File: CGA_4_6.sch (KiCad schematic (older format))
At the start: 3 parts, among them U1 74S112, U26 74S04, U47 74LS51

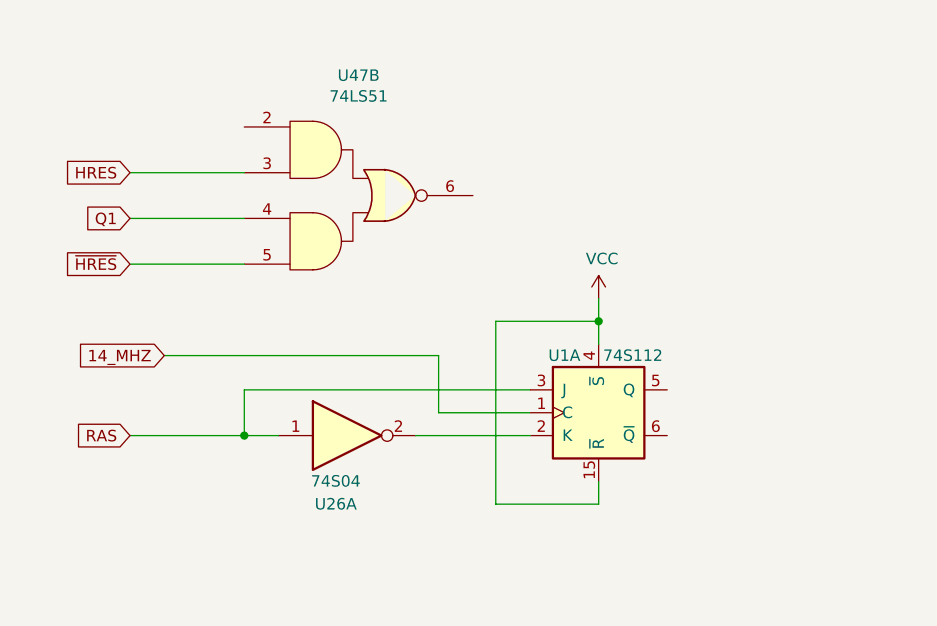
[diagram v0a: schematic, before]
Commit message: More CGA sheet 4
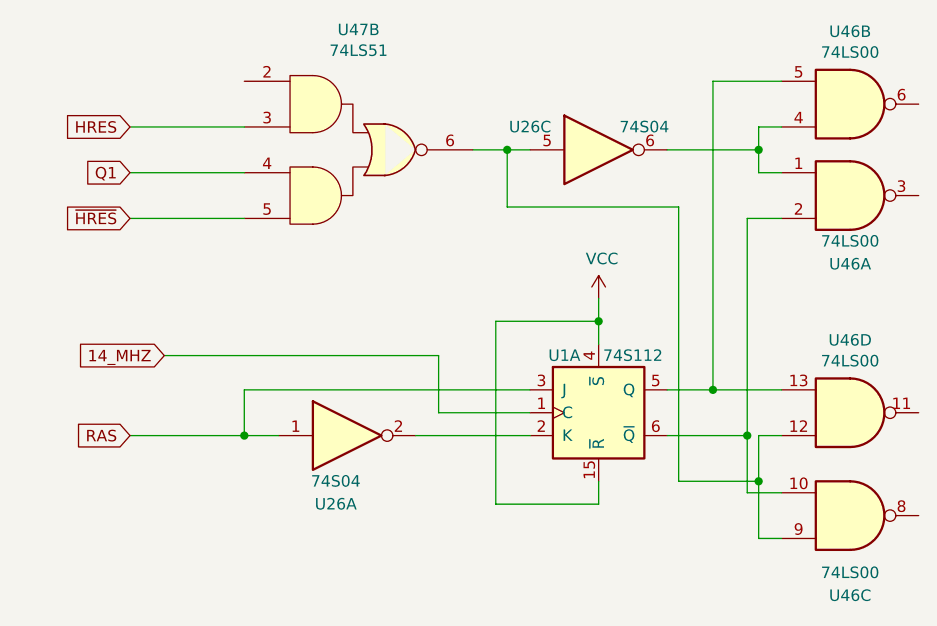
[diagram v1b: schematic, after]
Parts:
- added unit 3 of U26
- added U46: 74LS00, Package_DIP:DIP-14_W7.62mm_LongPads, symbol 74xx:74LS00
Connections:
- net at U47.6: now also U26.5, U46.12, U46.9
- net at U1.5 (Q): now also U46.13, U46.5
- net at U1.6 (~Q): now also U46.10, U46.2
- new net: U26.6, U46.1, U46.4
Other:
- moved on the sheet: U47B
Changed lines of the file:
@@
 L 74xx:74LS51 U47
 U 2 1 62D15655
-P 1850 1400
-F 0 "U47" H 1850 1925 50  0000 C CNN
-F 1 "74LS51" H 1850 1834 50  0000 C CNN
-F 2 "Package_DIP:DIP-14_W7.62mm_LongPads" H 1850 1400 50  0001 C CNN
-F 3 "http://www.ti.com/lit/ds/symlink/sn74ls51.pdf" H 1850 1400 50  0001 C CNN
-	2    1850 1400
-	1    0    0    -1
-$EndComp
+P 1850 1200
+F 0 "U47" H 1850 1725 50  0000 C CNN
+F 1 "74LS51" H 1850 1634 50  0000 C CNN
+F 2 "Package_DIP:DIP-14_W7.62mm_LongPads" H 1850 1200 50  0001 C CNN
+F 3 "http://www.ti.com/lit/ds/symlink/sn74ls51.pdf" H 1850 1200 50  0001 C CNN
+	2    1850 1200
+	1    0    0    -1
+$EndComp
+Wire Wire Line
+	1350 1100 850  1100
+Text GLabel 850  1100 0    50   Input ~ 0
+HRES
 Wire Wire Line
 	1350 1300 850  1300
 Text GLabel 850  1300 0    50   Input ~ 0
-HRES
+Q1
 Wire Wire Line
 	1350 1500 850  1500
 Text GLabel 850  1500 0    50   Input ~ 0
-Q1
-Wire Wire Line
-	1350 1700 850  1700
-Text GLabel 850  1700 0    50   Input ~ 0
 ~HRES
 $Comp
@@
 	2900 1950 2900 1850
 Connection ~ 2900 1950
+$Comp
+L 74xx:74LS04 U?
+U 3 1 62D569A0
+P 2900 1200
+AR Path="/60463C57/62D569A0" Ref="U?"  Part="2"
+AR Path="/60463CC5/62D569A0" Ref="U26"  Part="3"
+F 0 "U26" H 2600 1300 50  0000 C CNN
+F 1 "74S04" H 3100 1300 50  0000 C CNN
+F 2 "Package_DIP:DIP-14_W7.62mm_LongPads" H 2900 1200 50  0001 C CNN
+F 3 "http://www.ti.com/lit/gpn/sn74LS04" H 2900 1200 50  0001 C CNN
+	3    2900 1200
+	1    0    0    -1
+$EndComp
+Wire Wire Line
+	2350 1200 2500 1200
+$Comp
+L 74xx:74LS00 U46
+U 1 1 62D5F730
+P 4000 1400
+F 0 "U46" H 4000 1100 50  0000 C CNN
+F 1 "74LS00" H 4000 1200 50  0000 C CNN
+F 2 "Package_DIP:DIP-14_W7.62mm_LongPads" H 4000 1400 50  0001 C CNN
+F 3 "http://www.ti.com/lit/gpn/sn74ls00" H 4000 1400 50  0001 C CNN
+	1    4000 1400
+	1    0    0    -1
+$EndComp
+$Comp
+L 74xx:74LS00 U46
+U 2 1 62D5E238
+P 4000 1000
+F 0 "U46" H 4000 683 50  0000 C CNN
+F 1 "74LS00" H 4000 774 50  0000 C CNN
+F 2 "Package_DIP:DIP-14_W7.62mm_LongPads" H 4000 1000 50  0001 C CNN
+F 3 "http://www.ti.com/lit/gpn/sn74ls00" H 4000 1000 50  0001 C CNN
+	2    4000 1000
+	1    0    0    1
+$EndComp
+Wire Wire Line
+	3700 1100 3600 1100
+Wire Wire Line
+	3600 1100 3600 1200
+Wire Wire Line
+	3600 1300 3700 1300
+Wire Wire Line
+	3600 1200 3200 1200
+Connection ~ 3600 1200
+Wire Wire Line
+	3600 1200 3600 1300
+Wire Wire Line
+	3200 2250 3400 2250
+Wire Wire Line
+	3400 2250 3400 900
+Wire Wire Line
+	3400 900  3700 900
+Wire Wire Line
+	3200 2450 3550 2450
+Wire Wire Line
+	3550 2450 3550 1500
+Wire Wire Line
+	3550 1500 3700 1500
+$Comp
+L 74xx:74LS00 U46
+U 3 1 62D70773
+P 4000 2800
+F 0 "U46" H 4000 3150 50  0000 C CNN
+F 1 "74LS00" H 4000 3050 50  0000 C CNN
+F 2 "Package_DIP:DIP-14_W7.62mm_LongPads" H 4000 2800 50  0001 C CNN
+F 3 "http://www.ti.com/lit/gpn/sn74ls00" H 4000 2800 50  0001 C CNN
+	3    4000 2800
+	1    0    0    1
+$EndComp
+$Comp
+L 74xx:74LS00 U46
+U 4 1 62D6A442
+P 4000 2350
+F 0 "U46" H 4000 2033 50  0000 C CNN
+F 1 "74LS00" H 4000 2124 50  0000 C CNN
+F 2 "Package_DIP:DIP-14_W7.62mm_LongPads" H 4000 2350 50  0001 C CNN
+F 3 "http://www.ti.com/lit/gpn/sn74ls00" H 4000 2350 50  0001 C CNN
+	4    4000 2350
+	1    0    0    1
+$EndComp
+Wire Wire Line
+	3700 2250 3400 2250
+Connection ~ 3400 2250
+Wire Wire Line
+	3550 2450 3550 2700
+Wire Wire Line
+	3550 2700 3700 2700
+Connection ~ 3550 2450
+Wire Wire Line
+	3700 2450 3600 2450
+Wire Wire Line
+	3600 2450 3600 2650
+Wire Wire Line
+	3600 2900 3700 2900
+Wire Wire Line
+	3600 2650 3250 2650
+Wire Wire Line
+	3250 2650 3250 1450
+Wire Wire Line
+	3250 1450 2500 1450
+Wire Wire Line
+	2500 1450 2500 1200
+Connection ~ 3600 2650
+Wire Wire Line
+	3600 2650 3600 2900
+Connection ~ 2500 1200
+Wire Wire Line
+	2500 1200 2600 1200
 $EndSCHEMATC
